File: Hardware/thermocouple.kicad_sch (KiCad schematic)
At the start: 9 parts, among them U6 MAX31856

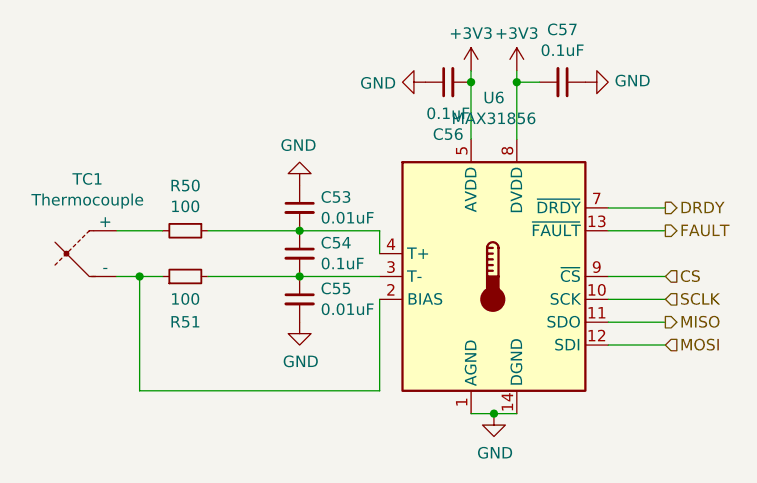
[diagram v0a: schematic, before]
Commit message: layout
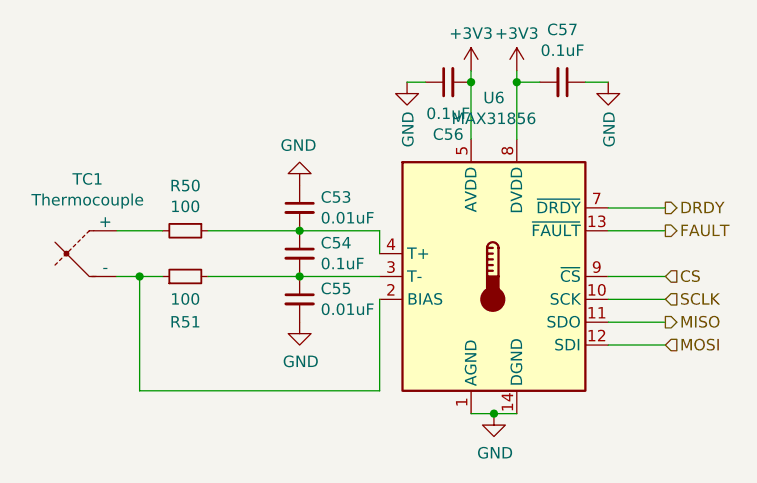
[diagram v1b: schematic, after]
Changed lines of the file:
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@@
+	(wire
+		(pts
+			(xy 105.41 52.07) (xy 107.95 52.07)
+		)
+		(stroke
+			(width 0)
+			(type default)
+		)
+	)
 	(wire
 		(pts
@@
 		(pts
 			(xy 63.5 68.58) (xy 73.66 68.58)
+		)
+		(stroke
+			(width 0)
+			(type default)
+		)
+	)
+	(wire
+		(pts
+			(xy 85.598 52.07) (xy 87.63 52.07)
 		)
 		(stroke
@@
 	(symbol
 		(lib_id "power:GND")
-		(at 87.63 52.07 270)
+		(at 85.598 52.07 0)
 		(unit 1)
 		(exclude_from_sim no)
@@
 		(dnp no)
 		(property "Reference" "#PWR0111"
-			(at 81.28 52.07 0)
+			(at 85.598 58.42 0)
 			(effects
 				(font
@@
 		)
 		(property "Value" "GND"
-			(at 84.3788 52.197 90)
+			(at 85.725 55.3212 90)
 			(effects
 				(font
@@
 		)
 		(property "Footprint" ""
-			(at 87.63 52.07 0)
+			(at 85.598 52.07 0)
 			(effects
 				(font
@@
 		)
 		(property "Datasheet" ""
-			(at 87.63 52.07 0)
-			(effects
-				(font
-					(size 1.27 1.27)
-				)
-				(hide yes)
-			)
-		)
-		(property "Description" ""
-			(at 87.63 52.07 0)
+			(at 85.598 52.07 0)
+			(effects
+				(font
+					(size 1.27 1.27)
+				)
+				(hide yes)
+			)
+		)
+		(property "Description" ""
+			(at 85.598 52.07 0)
 			(effects
 				(font
@@
 	(symbol
 		(lib_id "power:GND")
-		(at 105.41 52.07 90)
+		(at 107.95 52.07 0)
 		(unit 1)
 		(exclude_from_sim no)
@@
 		(dnp no)
 		(property "Reference" "#PWR0115"
-			(at 111.76 52.07 0)
+			(at 107.95 58.42 0)
 			(effects
 				(font
@@
 		)
 		(property "Value" "GND"
-			(at 108.6612 51.943 90)
+			(at 108.077 55.3212 90)
 			(effects
 				(font
@@
 		)
 		(property "Footprint" ""
-			(at 105.41 52.07 0)
+			(at 107.95 52.07 0)
 			(effects
 				(font
@@
 		)
 		(property "Datasheet" ""
-			(at 105.41 52.07 0)
-			(effects
-				(font
-					(size 1.27 1.27)
-				)
-				(hide yes)
-			)
-		)
-		(property "Description" ""
-			(at 105.41 52.07 0)
-			(effects
-				(font
+			(at 107.95 52.07 0)
+			(effects
+				(font
+					(size 1.27 1.27)
+				)
+				(hide yes)
+			)
+		)
+		(property "Description" ""
+			(at 107.95 52.07 0)
+			(effects
+				(font

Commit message: post Andrei review, new SD
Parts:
- TC1: footprint TerminalBlock_TE-Connectivity:TerminalBlock_TE_282834-2_1x02_P2.54mm_Horizontal -> Connector_Molex:Molex_Nano-Fit_105313-xx02_1x02_P2.50mm_Horizontal
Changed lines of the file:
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@@
 			)
 		)
-		(property "Footprint" "TerminalBlock_TE-Connectivity:TerminalBlock_TE_282834-2_1x02_P2.54mm_Horizontal"
+		(property "Footprint" "Connector_Molex:Molex_Nano-Fit_105313-xx02_1x02_P2.50mm_Horizontal"
 			(at 36.195 69.85 0)
 			(effects

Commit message: updated jumpers and silkscreen labelling
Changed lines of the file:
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@@
 (kicad_sch
-	(version 20231120)
+	(version 20250114)
 	(generator "eeschema")
-	(generator_version "8.0")
+	(generator_version "9.0")
 	(paper "A4")
 	(junction
@@
 		(shape input)
 		(at 114.3 81.28 0)
-		(fields_autoplaced yes)
 		(effects
 			(font
@@
 		(shape output)
 		(at 114.3 78.74 0)
-		(fields_autoplaced yes)
 		(effects
 			(font
@@
 		(shape output)
 		(at 114.3 68.58 0)
-		(fields_autoplaced yes)
 		(effects
 			(font
@@
 		(shape input)
 		(at 114.3 73.66 0)
-		(fields_autoplaced yes)
 		(effects
 			(font
@@
 		(shape output)
 		(at 114.3 66.04 0)
-		(fields_autoplaced yes)
 		(effects
 			(font
@@
 		(shape input)
 		(at 114.3 76.2 0)
-		(fields_autoplaced yes)
-		(effects
-			(font
+		(effects
+			(font

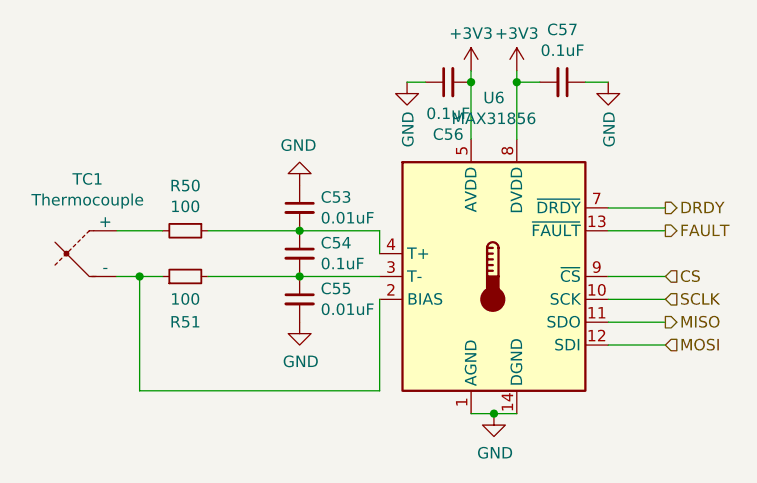
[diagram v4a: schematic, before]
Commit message: tidy up schematic and bom
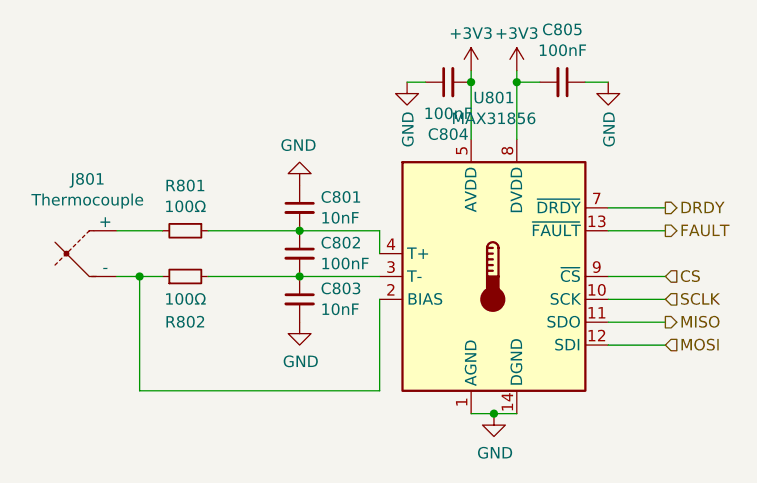
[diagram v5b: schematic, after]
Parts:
- C801: renamed from C53; value 0.01uF -> 10nF
- C802: renamed from C54; value 0.1uF -> 100nF
- C803: renamed from C55; value 0.01uF -> 10nF
- C804: renamed from C56; value 0.1uF -> 100nF
- C805: renamed from C57; value 0.1uF -> 100nF
- R801: renamed from R50; value 100 -> 100Ω
- R802: renamed from R51; value 100 -> 100Ω
- renumbered TC1 to J801, U6 to U801
